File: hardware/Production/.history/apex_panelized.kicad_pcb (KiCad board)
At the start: 2 copper layers, 43.1 x 46.6 mm, 35 parts, among them IC1 FE1.1S, J1 USB_C_Receptacle_USB2.0_16P, J2 USB_A, J3 USB_A, U1 USBLC6-2SC6, U2 USBLC6-2SC6, U3 USBLC6-2SC6, Y2 Crystal

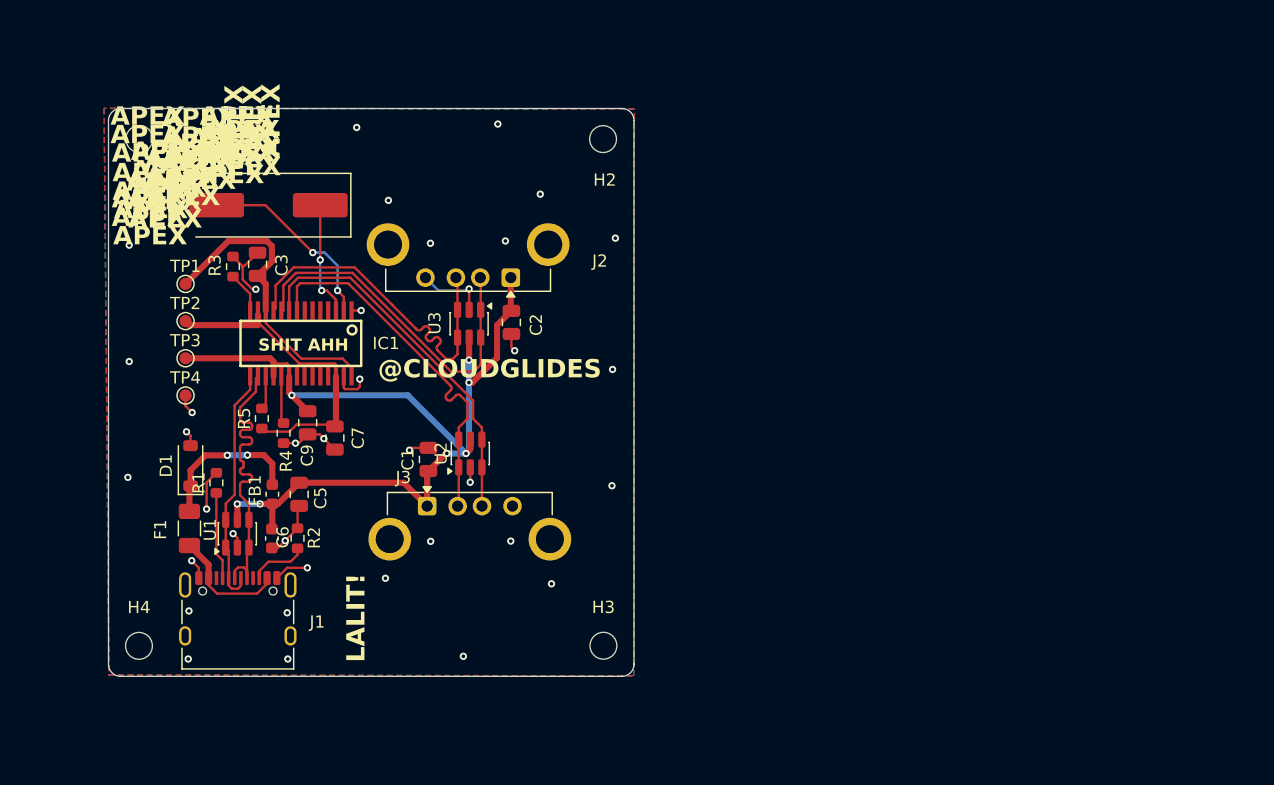
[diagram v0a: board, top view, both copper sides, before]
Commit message: revise: apex_2
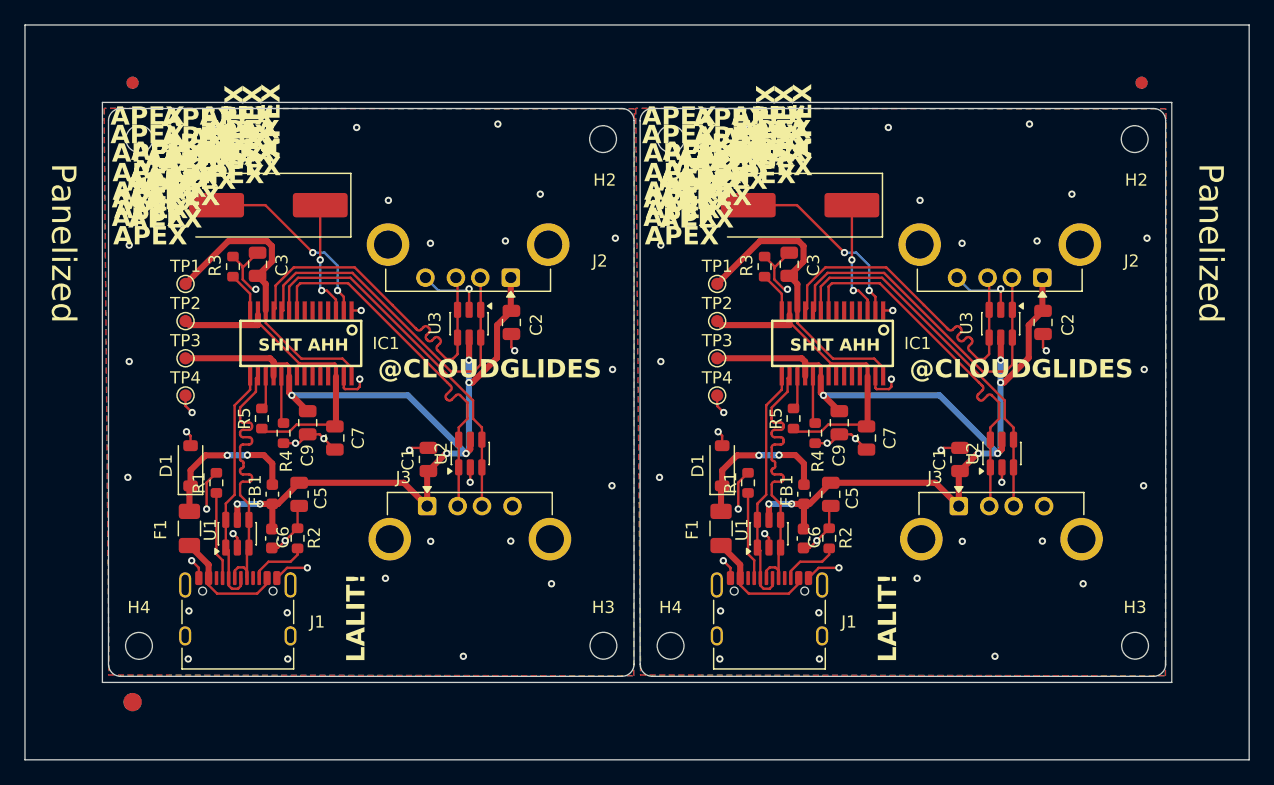
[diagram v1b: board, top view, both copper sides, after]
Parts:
- added ?: , Fiducial_1mm_Mask3mm, F.Cu at (207.9, 67.8)
- added ?: , Fiducial_1.5mm_Mask3mm, F.Cu at (125.2, 118.6)
- added ?: , Fiducial_1mm_Mask3mm, F.Cu at (125.2, 67.8)
- added ?: , Fiducial_1mm_Mask3mm, B.Cu at (207.9, 67.8)
- added ?: , Fiducial_1mm_Mask3mm, B.Cu at (125.2, 67.8)
- added ?: , Fiducial_1.5mm_Mask3mm, B.Cu at (125.2, 118.6)
- added C1: 10uf, Capacitor_SMD:C_0805_2012Metric, F.Cu at (193.1, 98.7)
- added C2: 10uf, Capacitor_SMD:C_0805_2012Metric, F.Cu at (199.9, 87.4)
- added C3: 10uf, Capacitor_SMD:C_0805_2012Metric, F.Cu at (179.0, 82.7)
- added C5: 4.7uf, Capacitor_SMD:C_0805_2012Metric, F.Cu at (182.4, 101.5)
- added C6: 100nf, Capacitor_SMD:C_0603_1608Metric, F.Cu at (180.2, 105.1)
- added C7: 10uf, Capacitor_SMD:C_0805_2012Metric, F.Cu at (185.4, 96.9)
- added C9: 10uf, Capacitor_SMD:C_0805_2012Metric, F.Cu at (183.2, 95.7)
- added D1: 5V, Diode_SMD:D_SOD-123, F.Cu at (173.5, 99.2)
- added F1: Polyfuse, Fuse:Fuse_1206_3216Metric, F.Cu at (173.4, 104.3)
- added FB1: 220Ω@100MHz, Inductor_SMD:L_0603_1608Metric, F.Cu at (180.2, 101.5)
- added G***: LOGO, LOGO, B.Cu at (176.0, 79.7)
- added G***: LOGO, LOGO, B.Cu at (177.3, 104.7)
- added G***: LOGO, LOGO, B.Cu at (197.3, 105.9)
- added G***: LOGO, LOGO, B.Cu at (199.2, 81.5)
- added H1: MountingHole, MountingHole:MountingHole_2.2mm_M2, F.Cu at (169.3, 72.4)
- added H2: MountingHole, MountingHole:MountingHole_2.2mm_M2, F.Cu at (207.4, 72.4)
- added H3: MountingHole, MountingHole:MountingHole_2.2mm_M2, F.Cu at (207.4, 113.9)
- added H4: MountingHole, MountingHole:MountingHole_2.2mm_M2, F.Cu at (169.3, 114.0)
- added IC1: FE1.1S, fe1.1s:FE1.1S_SSOP-28, F.Cu at (182.6, 89.1)
- added J1: USB_C_Receptacle_USB2.0_16P, Connector_USB:USB_C_Receptacle_XKB_U262-16XN-4BVC11, F.Cu at (177.4, 112.1)
- added J2: USB_A, Connector_USB:USB_A_Connfly_DS1095, F.Cu at (199.8, 83.7)
- added J3: USB_A, Connector_USB:USB_A_Connfly_DS1095, F.Cu at (192.9, 102.5)
- added R1: 5.1K, Resistor_SMD:R_0603_1608Metric, F.Cu at (175.7, 100.6)
- added R2: 5.1K, Resistor_SMD:R_0603_1608Metric, F.Cu at (182.3, 105.1)
- added R3: 2.7K, Resistor_SMD:R_0603_1608Metric, F.Cu at (177.0, 82.8)
- added R4: 10K, Resistor_SMD:R_0603_1608Metric, F.Cu at (181.2, 96.5)
- added R5: 10K, Resistor_SMD:R_0603_1608Metric, F.Cu at (179.4, 95.3)
- added TP1: TestPoint, TestPoint:TestPoint_Pad_D1.0mm, F.Cu at (173.1, 84.3)
- added TP2: TestPoint, TestPoint:TestPoint_Pad_D1.0mm, F.Cu at (173.1, 87.3)
- added TP3: TestPoint, TestPoint:TestPoint_Pad_D1.0mm, F.Cu at (173.1, 90.4)
- added TP4: TestPoint, TestPoint:TestPoint_Pad_D1.0mm, F.Cu at (173.1, 93.4)
- added U1: USBLC6-2SC6, Package_TO_SOT_SMD:SOT-23-6, F.Cu at (177.4, 104.8)
- added U2: USBLC6-2SC6, Package_TO_SOT_SMD:SOT-23-6, F.Cu at (196.5, 98.2)
- added U3: USBLC6-2SC6, Package_TO_SOT_SMD:SOT-23-6, F.Cu at (196.4, 87.5)
- added Y2: Crystal, Crystal:Crystal_SMD_HC49-SD, F.Cu at (179.9, 77.8)
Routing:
- net VBUS: track 79.5 -> 159.0 mm, vias 7 -> 14
- net GND: track 41.0 -> 82.0 mm, vias 38 -> 76
- net USB2_DP: track 30.5 -> 60.9 mm
- net USB2_DN: track 30.4 -> 60.7 mm
- net USB1_DN: track 29.5 -> 59.1 mm
- net USB1_DP: track 29.3 -> 58.6 mm
- net +3V3: track 27.7 -> 55.3 mm
- net +1V8: track 25.0 -> 50.1 mm
- net USB_UP_DP: track 24.6 -> 49.1 mm
- net USB_UP_DN: track 19.9 -> 39.9 mm
- net /xo: track 15.9 -> 31.7 mm, vias 2 -> 4
- net Net-(D1-A1): track 12.5 -> 25.0 mm, vias 2 -> 4
- net /xi: track 9.42 -> 18.8 mm, vias 2 -> 4
- net Net-(F1-Pad2): track 9.32 -> 18.6 mm
- net Net-(J1-CC1): track 7.20 -> 14.4 mm
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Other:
- board size 43.1 x 46.6 mm -> 100.4 x 60.3 mm
- board text added: "Panelized"
- board text added: "V-SCORE"
